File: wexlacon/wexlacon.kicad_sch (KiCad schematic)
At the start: 18 parts, among them J1 CAN25, J2 Screw_Terminal_01x02, J3 Screw_Terminal_01x03, J4 Screw_Terminal_01x03, J5 Conn_01x04, J6 Conn_01x02, J7 Conn_01x02, J8 Conn_01x02

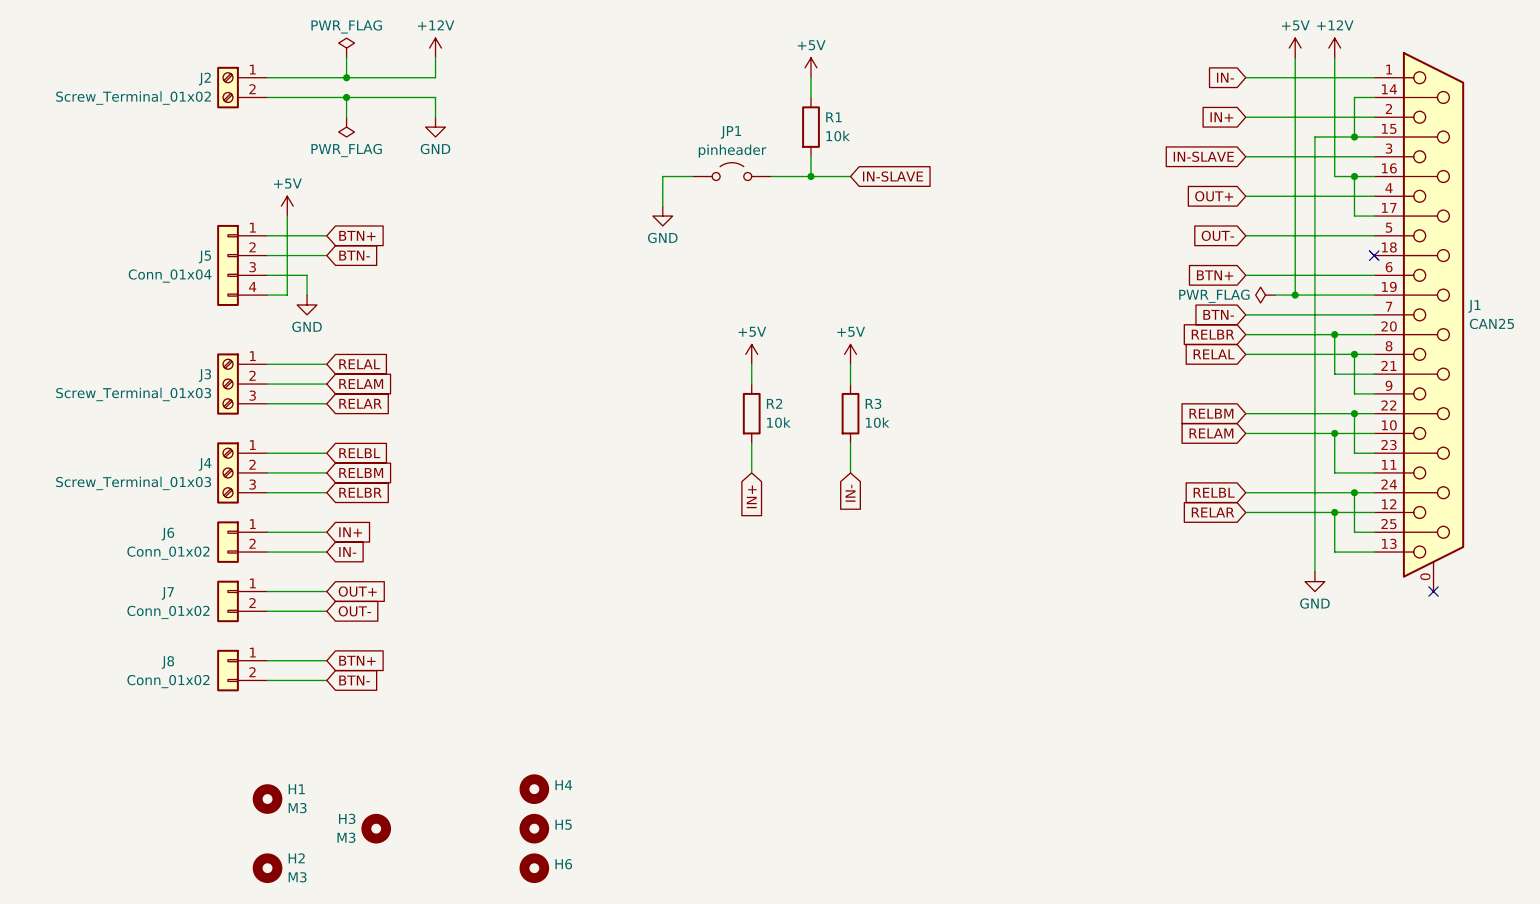
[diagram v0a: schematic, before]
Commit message: wexlacon: pcb.
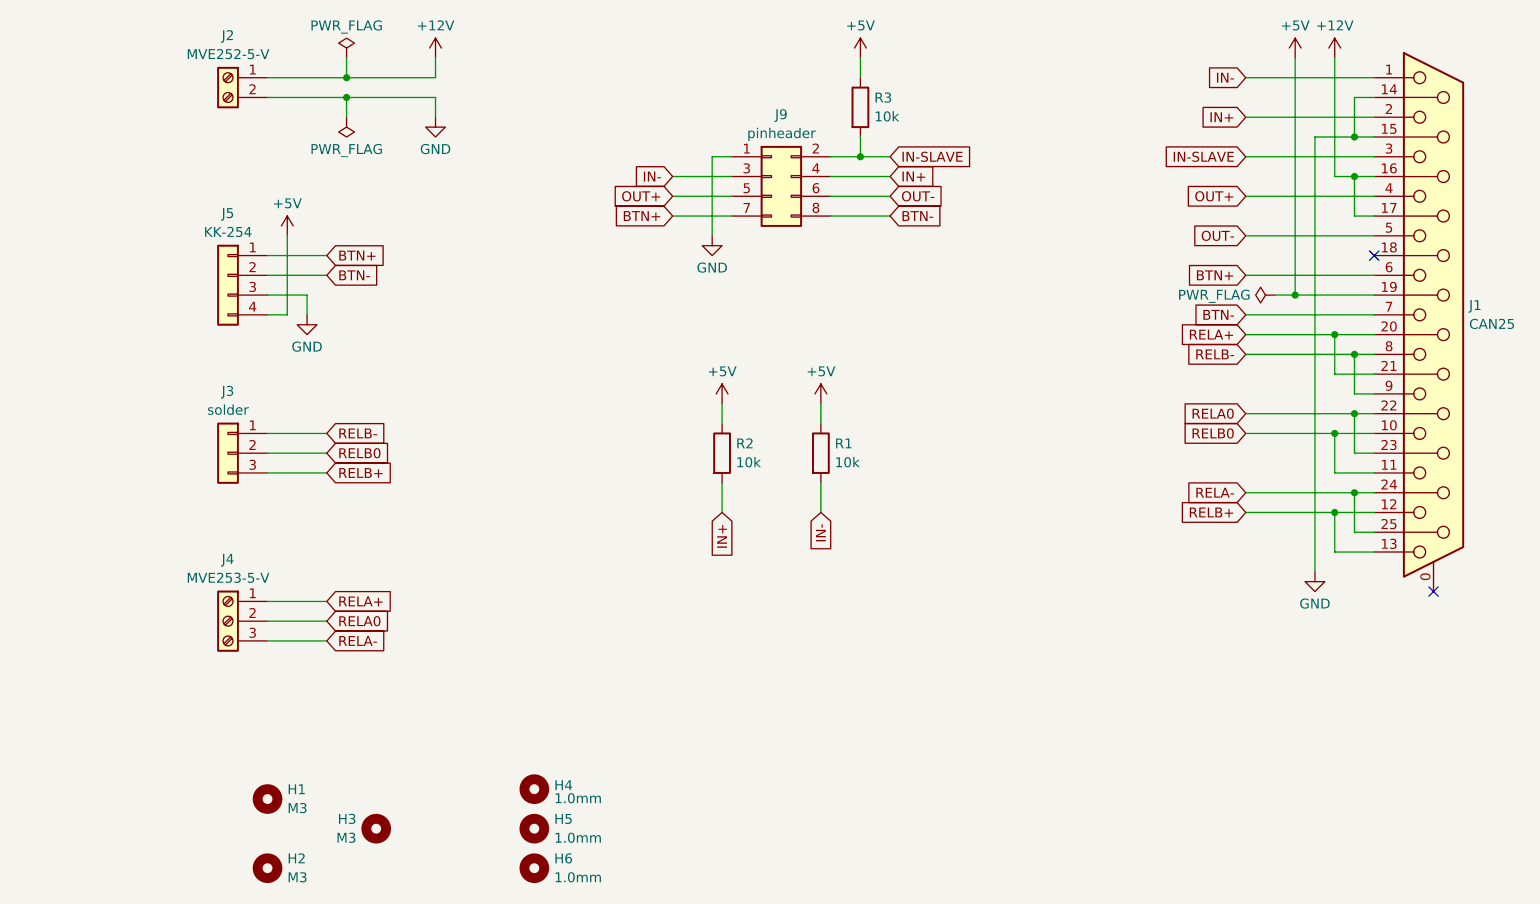
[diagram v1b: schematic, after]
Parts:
- removed J6, J7, J8: Conn_01x02, symbol Connector_Generic:Conn_01x02
- removed JP1: pinheader, Connector_PinHeader_2.54mm:PinHeader_1x02_P2.54mm_Vertical, symbol Jumper:Jumper_2_Open
- added J9: pinheader, Connector_PinHeader_2.54mm:PinHeader_2x04_P2.54mm_Vertical, symbol Connector_Generic:Conn_02x04_Odd_Even
- H4, H5, H6: value ~ -> 1.0mm; footprint (none) -> TestPoint:TestPoint_THTPad_D2.0mm_Drill1.0mm
- J1: footprint Connector_Dsub:DSUB-25_Female_Vertical_P2.77x2.84mm_MountingHoles -> Connector_Dsub:DSUB-25_Female_Vertical_P2.77x2.84mm
- J2: value Screw_Terminal_01x02 -> MVE252-5-V; footprint (none) -> TerminalBlock_Euroclamp:MVE252-5-V
- J3: value Screw_Terminal_01x03 -> solder; footprint (none) -> relaycon:RELAYCON; symbol Connector:Screw_Terminal_01x03 -> Connector_Generic:Conn_01x03
- J4: value Screw_Terminal_01x03 -> MVE253-5-V; footprint (none) -> relaycon:RELAYCON
- J5: value Conn_01x04 -> KK-254
- R1: renamed from R3; footprint Resistor_SMD:R_1206_3216Metric -> Resistor_SMD:R_1206_3216Metric_Pad1.30x1.75mm_HandSolder
- R2: footprint Resistor_SMD:R_1206_3216Metric -> Resistor_SMD:R_1206_3216Metric_Pad1.30x1.75mm_HandSolder
- R3: renamed from R1; footprint Resistor_SMD:R_1206_3216Metric -> Resistor_SMD:R_1206_3216Metric_Pad1.30x1.75mm_HandSolder
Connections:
- net BTN+: now also J9.7 (Pin_7)
- net BTN-: now also J9.8 (Pin_8)
- net GND: now also J9.1 (Pin_1)
- net IN+: now also J9.4 (Pin_4)
- net IN-: now also J9.3 (Pin_3)
- net IN-SLAVE: now also J9.2 (Pin_2)
- net OUT+: now also J9.5 (Pin_5)
- net OUT-: now also J9.6 (Pin_6)
- net RELAL renamed RELB-
- net RELAM renamed RELB0
- net RELAR renamed RELB+
- net RELBL renamed RELA-
- net RELA-: now also J4.3 (Pin_3); no longer J4.1 (Pin_1)
- net RELBM renamed RELA0
- net RELBR renamed RELA+
- net RELA+: now also J4.1 (Pin_1); no longer J4.3 (Pin_3)
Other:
- moved on the sheet: J4, J5, R1, R2, R3
